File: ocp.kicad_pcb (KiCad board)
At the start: 2 copper layers, 54 x 54 mm, 13 parts, among them J1 ADS1115, J2 Screw_Terminal_01x03, J3 Screw_Terminal_01x02, U2 REF3033, U3 TL072

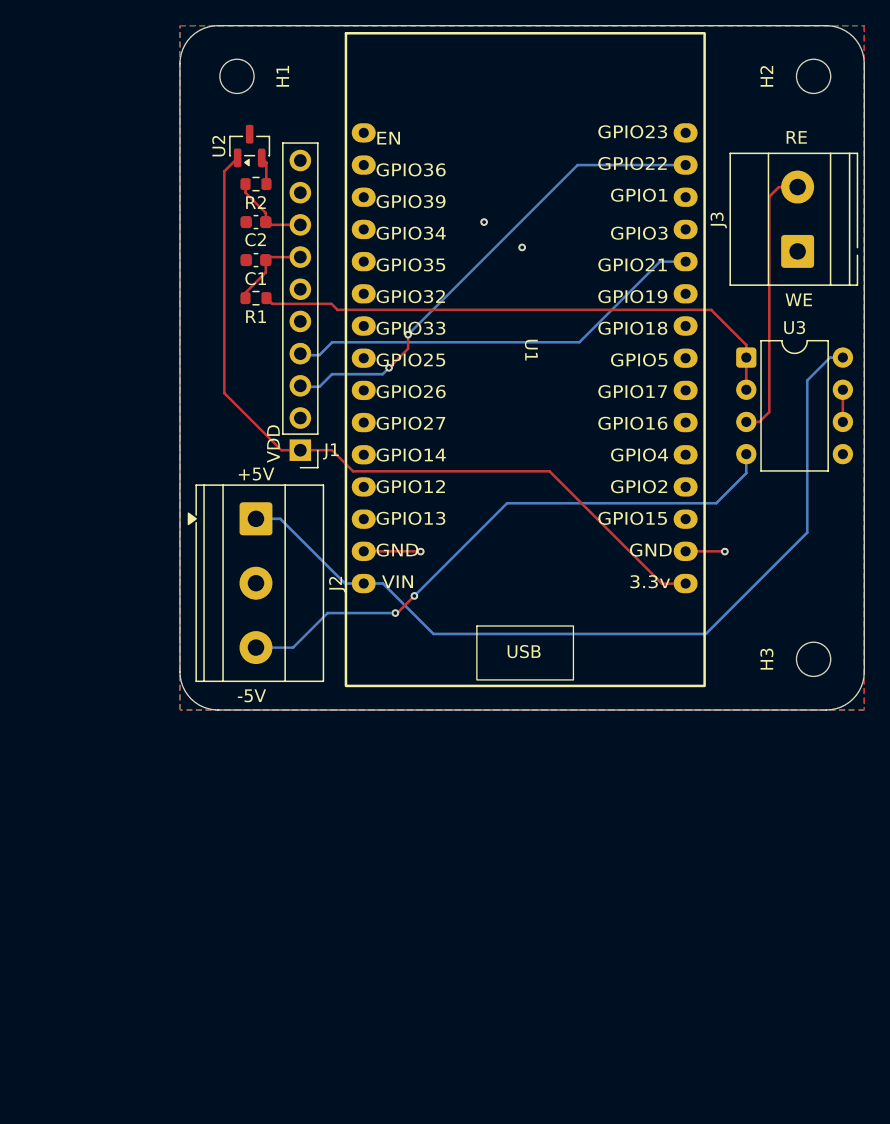
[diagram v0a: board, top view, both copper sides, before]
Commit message: Updated PCB
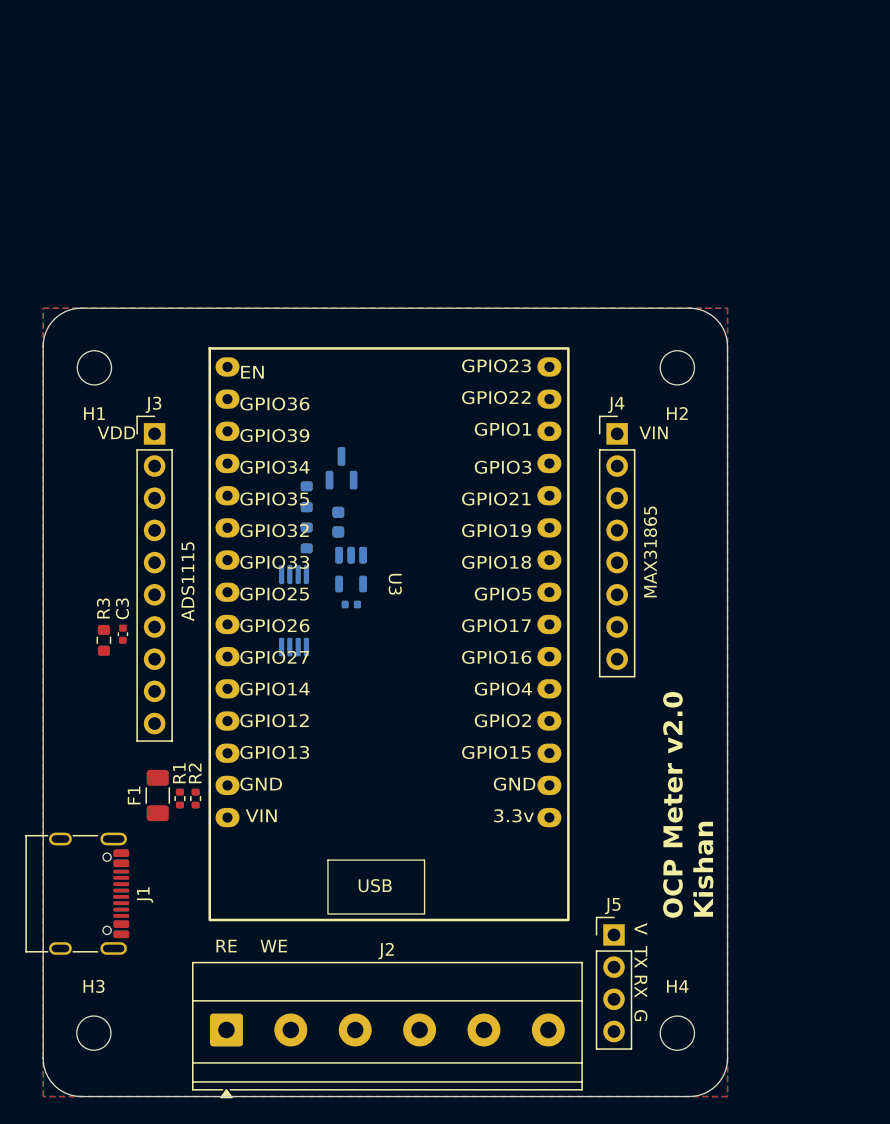
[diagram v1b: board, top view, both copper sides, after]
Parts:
- added C3: 1u, Capacitor_SMD:C_0402_1005Metric, F.Cu at (107.0, 125.0)
- added F1: 0.35A, Fuse:Fuse_1206_3216Metric, F.Cu at (109.8, 137.8)
- added H4: MountingHole, MountingHole:MountingHole_2.7mm_M2.5, F.Cu at (150.8, 156.5)
- added J4: MAX31865, Connector_PinHeader_2.54mm:PinHeader_1x08_P2.54mm_Vertical, F.Cu at (146.0, 109.2)
- added J5: UART, Connector_PinHeader_2.54mm:PinHeader_1x04_P2.54mm_Vertical, F.Cu at (145.8, 148.8)
- added R3: 100, Resistor_SMD:R_0603_1608Metric, F.Cu at (105.5, 125.5)
- added R4: 10k, Resistor_SMD:R_0603_1608Metric, B.Cu at (121.5, 117.4)
- added R5: 10k, Resistor_SMD:R_0603_1608Metric, B.Cu at (121.5, 114.2)
- added U4: TLV9062, Package_SO:TSSOP-8_4.4x3mm_P0.65mm, B.Cu at (120.5, 123.2)
- C1: footprint Capacitor_SMD:C_0603_1608Metric -> Capacitor_SMD:C_0402_1005Metric; moved to B.Cu
- C2: value 1u -> 2.2u; moved to B.Cu
- J1: value ADS1115 -> USB_C_Receptacle; footprint Connector_PinHeader_2.54mm:PinHeader_1x10_P2.54mm_Vertical -> Connector_USB:USB_C_Receptacle_G-Switch_GT-USB-7010ASV
- J2: value Screw_Terminal_01x03 -> Aviation_6Pin_GX16; footprint TerminalBlock_Phoenix:TerminalBlock_Phoenix_MKDS-1,5-3-5.08_1x03_P5.08mm_Horizontal -> TerminalBlock_Phoenix:TerminalBlock_Phoenix_MKDS-1,5-6-5.08_1x06_P5.08mm_Horizontal
- J3: value Screw_Terminal_01x02 -> ADS1115; footprint TerminalBlock_Phoenix:TerminalBlock_Phoenix_MKDS-1,5-2-5.08_1x02_P5.08mm_Horizontal -> Connector_PinHeader_2.54mm:PinHeader_1x10_P2.54mm_Vertical
- R1, R2: value 100 -> 5.1k; footprint Resistor_SMD:R_0603_1608Metric -> Resistor_SMD:R_0402_1005Metric
- U1: value ~ -> TPS60403DBV; footprint PCM_ESP32_30Pin:ESP32_30Pin -> Package_TO_SOT_SMD:SOT-23-5; moved to B.Cu
- U2: moved to B.Cu
- U3: value TL072 -> ESP32_30Pin; footprint Package_DIP:DIP-8_W7.62mm -> PCM_ESP32_30Pin:ESP32_30Pin
- moved H3 64.0 mm to (104.7, 156.5), turned to 0 degrees
- moved J3 52.7 mm to (109.5, 109.2), turned to 0 degrees
- moved R2 48.7 mm to (112.7, 138.0), turned to 90 degrees
- moved J2 40.4 mm to (115.2, 156.2), turned to 0 degrees
- moved R1 39.9 mm to (111.5, 138.0), turned to 90 degrees
- moved J1 39.3 mm to (103.1, 145.5), turned to -90 degrees
- moved U3 34.8 mm to (127.2, 122.5)
- moved C1 28.2 mm to (125.0, 122.7)
- moved U2 26.4 mm to (124.2, 111.9)
- moved H1 25.6 mm to (104.8, 104.0), turned to 180 degrees
- moved H2 25.4 mm to (150.8, 104.0), turned to 180 degrees
- moved C2 24.6 mm to (124.0, 116.2), turned to 90 degrees
- moved U1 20.5 mm to (125.0, 119.9), turned to -90 degrees
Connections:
- C1 pad 1: GND -> Net-(U1-C_{FLY+})
- C1 pad 2: Net-(J1-Pin_7) -> Net-(U1-C_{FLY-})
- C2 pad 1: Net-(J1-Pin_8) -> -3V3
- J2 pad 1: +5V -> GND
- J2 pad 2: GND -> /WE
- J2 pad 3: -5V -> unconnected-(J2-Pin_3-Pad3)
- J3 pad 1: GND -> +3V3
- J3 pad 2: /V- -> GND
- R1 pad 1: Net-(J1-Pin_7) -> Net-(J1-CC1)
- R1 pad 2: /RE -> GND
- R2 pad 1: Net-(J1-Pin_8) -> Net-(J1-CC2)
- R2 pad 2: /VREF -> GND
- U1 pad 1: +5V -> -3V3
- U1 pad 2: GND -> /VREF
- U1 pad 3: unconnected-(U1-GPIO13-Pad3) -> Net-(U1-C_{FLY-})
- U1 pad 4: unconnected-(U1-GPIO12-Pad4) -> GND
- U1 pad 5: unconnected-(U1-GPIO14-Pad5) -> Net-(U1-C_{FLY+})
- U3 pad 1: /RE -> +5V
- U3 pad 2: /RE -> GND
- U3 pad 3: /V- -> unconnected-(U3-GPIO13-Pad3)
- U3 pad 4: -5V -> unconnected-(U3-GPIO12-Pad4)
- U3 pad 5: GND -> unconnected-(U3-GPIO14-Pad5)
- U3 pad 6: Net-(U3B--) -> unconnected-(U3-GPIO27-Pad6)
- U3 pad 7: Net-(U3B--) -> unconnected-(U3-GPIO26-Pad7)
- U3 pad 8: +5V -> unconnected-(U3-GPIO25-Pad8)
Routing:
- net +5V: track 66.1 -> 0.00 mm
- net +3V3: track 61.6 -> 0.00 mm
- net -5V: track 45.9 -> 0.00 mm, vias 2 -> 0
- net /RE: track 42.9 -> 0.00 mm
- net /SCL: track 38.3 -> 0.00 mm, vias 2 -> 0
- net /SDA: track 33.5 -> 0.00 mm
- net /V-: track 21.7 -> 0.00 mm
- net GND: track 7.61 -> 0.00 mm, vias 2 -> 0
- net Net-(J1-Pin_7): track 6.49 -> 0.00 mm
- net Net-(J1-Pin_8): track 6.48 -> 0.00 mm
- net Net-(U3B--): track 2.54 -> 0.00 mm
- net /VREF: track 2.22 -> 0.00 mm
- net (no net): vias 2 -> 0
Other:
- board size 54 x 54 mm -> 54 x 62.2 mm
- board text added: "ADS1115"
- board text added: "Indriya Sensotech Private Limited"
- board text added: "MAX31865"
- board text added: "OCP Meter v2.0 Kishan"
- board text added: "RE WE"
- board text added: "V TX RX G"
- board text added: "VIN"
- board text removed: "+5V"
- board text removed: "-5V"
- board text removed: "Indriya Sensotech Private Limited OCP Meter v1.0 Kishan"
- board text removed: "RE"
- board text removed: "WE"
